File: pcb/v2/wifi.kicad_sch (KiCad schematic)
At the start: 10 parts, among them U10 AIC8800

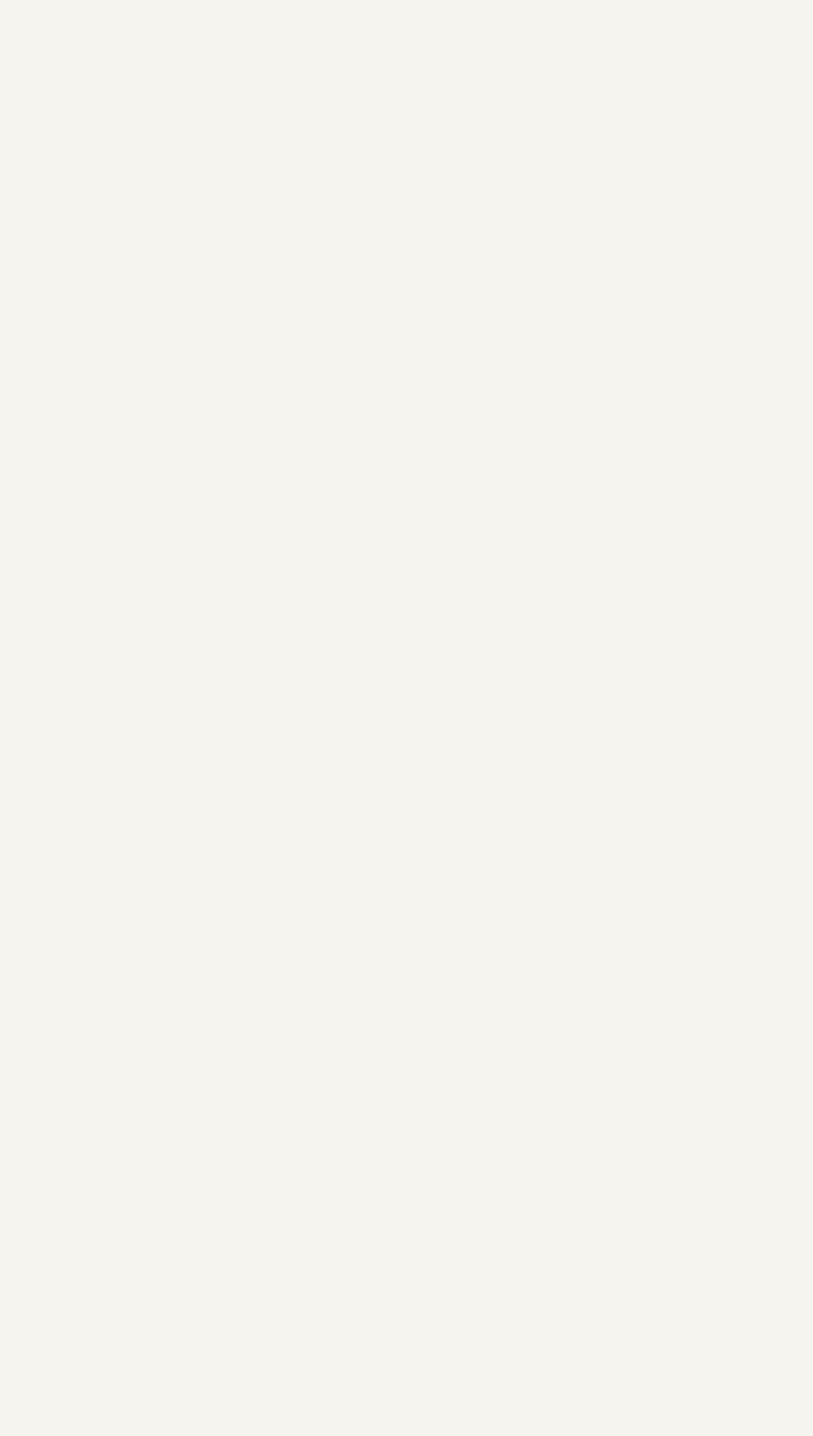
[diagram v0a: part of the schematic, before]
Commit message: up
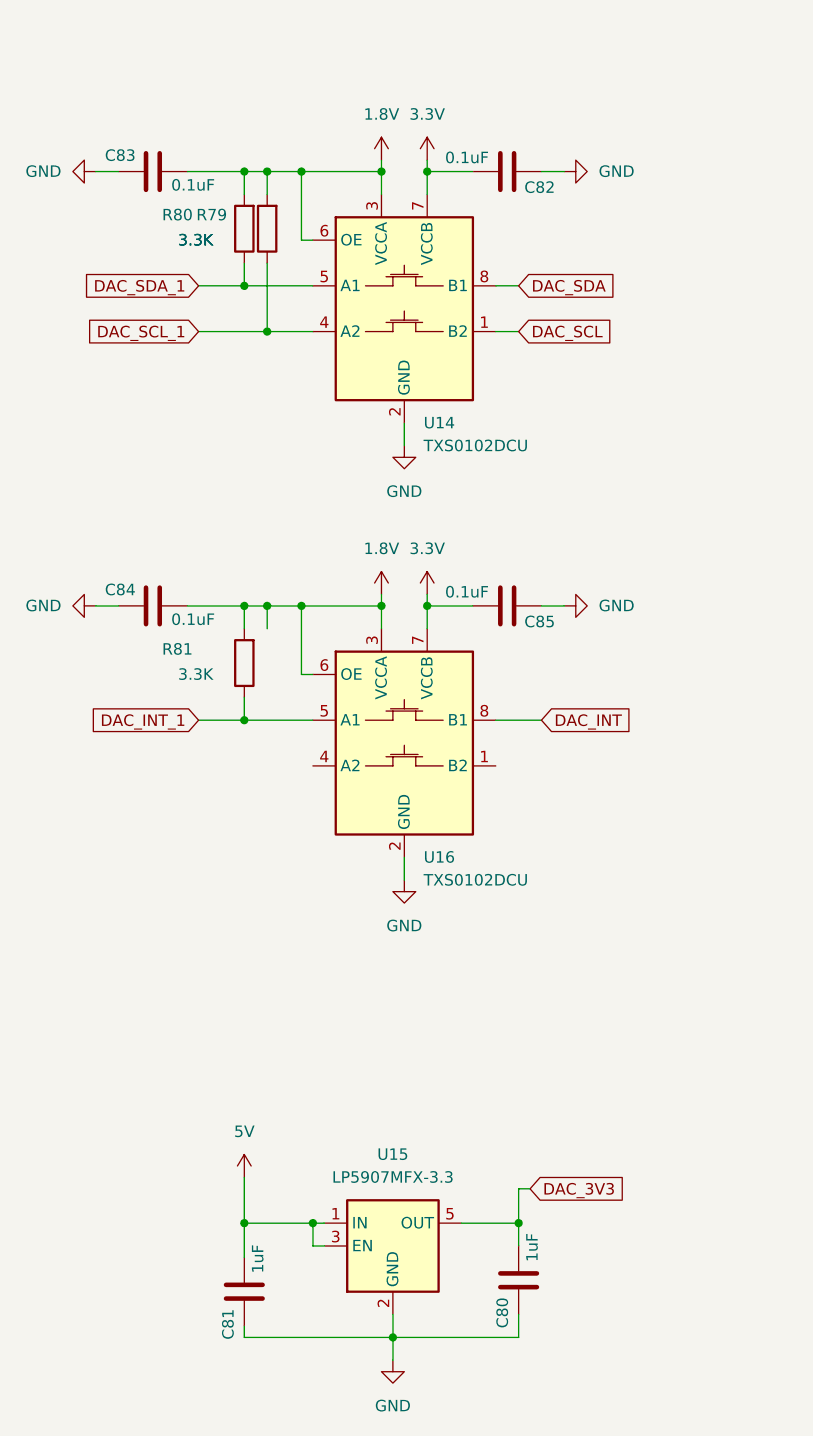
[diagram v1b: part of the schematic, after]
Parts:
- added C80, C81: 1uF, Capacitor_SMD:C_0402_1005Metric_Pad0.74x0.62mm_HandSolder, symbol Device:C
- added C82, C83, C84, C85: 0.1uF, Capacitor_SMD:C_0402_1005Metric_Pad0.74x0.62mm_HandSolder, symbol Device:C
- added R79, R80, R81: 3.3K, Capacitor_SMD:C_0402_1005Metric_Pad0.74x0.62mm_HandSolder, symbol Device:R
- added U14, U16: TXS0102DCU, Package_SO:VSSOP-8_2.3x2mm_P0.5mm, symbol Logic_LevelTranslator:TXS0102DCU
- added U15: LP5907MFX-3.3, Package_TO_SOT_SMD:SOT-23-5, symbol Regulator_Linear:LP5907MFX-3.3
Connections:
- net 3.3V: now also C82.1, C85.1, U14.7 (VCCB), U16.7 (VCCB)
- net GND: now also C80.2, C81.2, C82.2, C83.2, C84.2, C85.2, U14.2 (GND), U15.2 (GND), U16.2 (GND)
- new net 1.8V: C83.1, C84.1, R79.2, R80.2, R81.2, U14.3 (VCCA), U14.6 (OE), U16.3 (VCCA), U16.6 (OE)
- new net 5V: C81.1, U15.1 (IN), U15.3 (EN)
- new net DAC_3V3: C80.1, U15.5 (OUT)
- new net DAC_INT: U16.8 (B1)
- new net DAC_INT_1: R81.1, U16.5 (A1)
- new net DAC_SCL: U14.1 (B2)
- new net DAC_SCL_1: R79.1, U14.4 (A2)
- new net DAC_SDA: U14.8 (B1)
- new net DAC_SDA_1: R80.1, U14.5 (A1)
